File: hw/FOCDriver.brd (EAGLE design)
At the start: 99.1 x 68 mm, 103 parts, among them U1 IX4428N, U2 IX4428N, U3 IX4428N, U4 IRF9389TRPBF, U5 IRF9389TRPBF, U6 IRF9389TRPBF, U7 LM27313XMF, U8 MCP6024T-I, U9 TLV3201AIDBVR

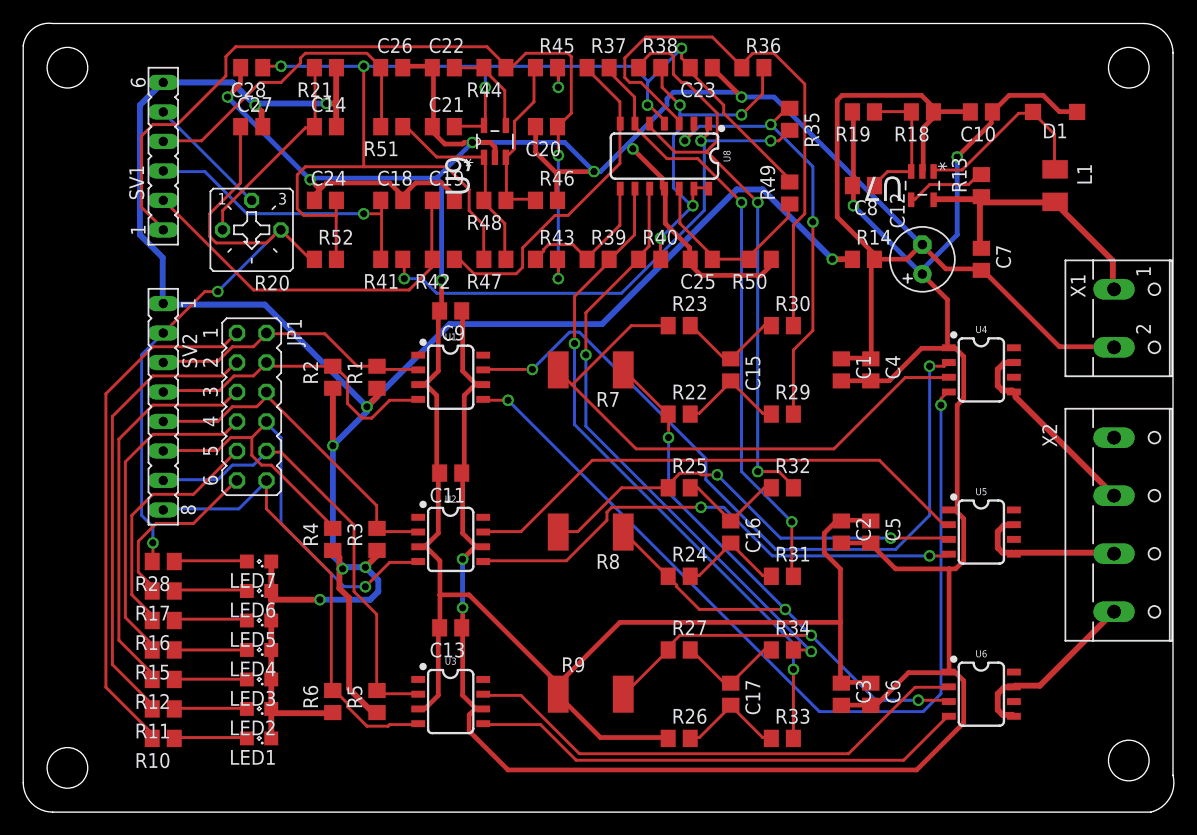
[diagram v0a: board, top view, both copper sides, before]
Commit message: layout
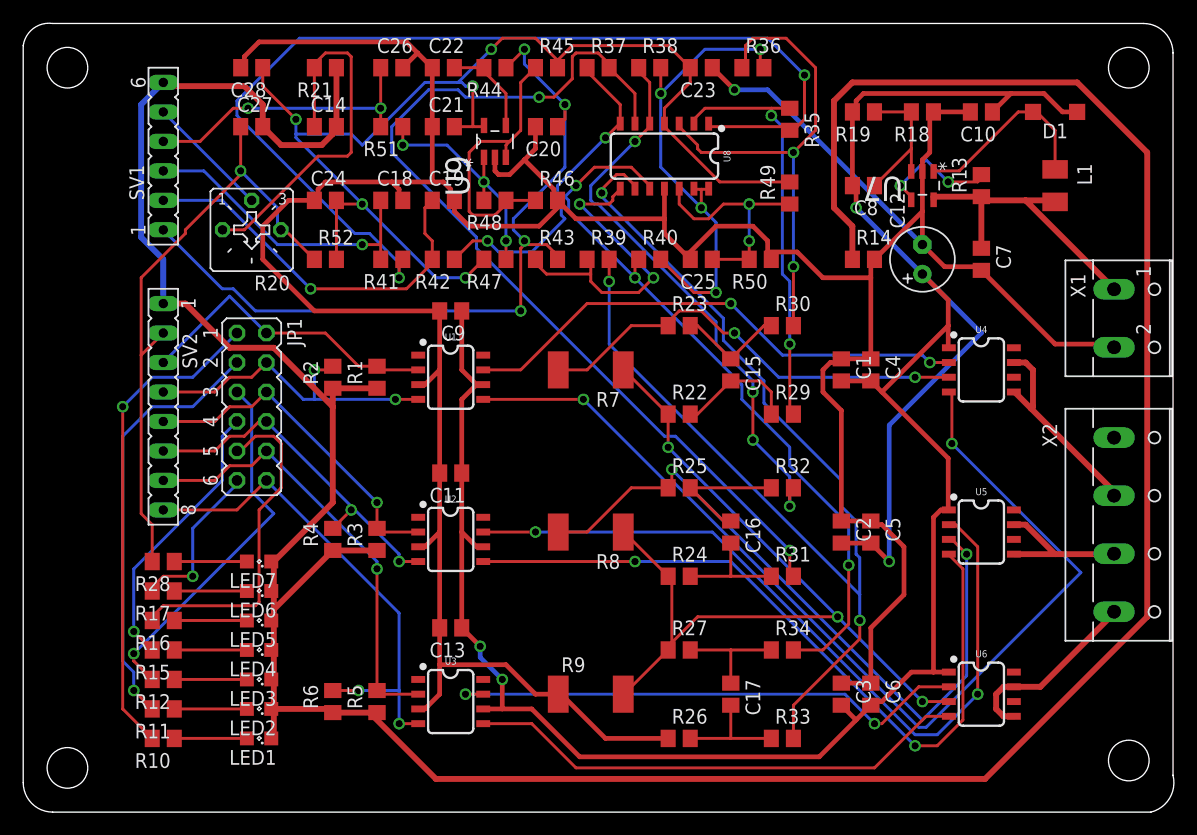
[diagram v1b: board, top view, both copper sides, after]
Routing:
- net GND: track 192.3 -> 281.4 mm, vias 8 -> 0
- net N$24: track 57.4 -> 100.8 mm, vias 2 -> 3
- net N$16: track 46.8 -> 89.0 mm, vias 3 -> 2
- net N$19: track 52.0 -> 83.5 mm
- net AGND: track 336.5 -> 312.9 mm, vias 7 -> 1
- net SHUNT_HIGH2: track 38.3 -> 61.4 mm
- net N$8: track 45.0 -> 67.3 mm, vias 0 -> 2
- net N$10: track 64.5 -> 44.6 mm
- net N$7: track 44.3 -> 63.7 mm
- net PWM1L2: track 45.6 -> 31.0 mm, vias 1 -> 2
- net N$26: track 13.0 -> 27.4 mm, vias 0 -> 2
- net N$29: track 17.7 -> 31.4 mm
- net N$25: track 51.8 -> 63.6 mm, vias 2 -> 3
- net N$9: track 77.6 -> 89.1 mm
- net SHUNT_HIGH1: track 49.5 -> 38.5 mm, vias 0 -> 2
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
